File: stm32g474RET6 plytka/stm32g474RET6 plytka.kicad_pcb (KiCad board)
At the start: 4 copper layers, 73.5 x 39 mm, 60 parts, among them IC1 STM32G484RET6, IC2 SN65HVD230DR, IC3 SN65HVD230DR, IC4 TPSM63603V3RDHR, IC5 ESP32-S3-WROOM-1-N8, J1 5055670431, J2 5055670631, J3 5055670631, J4 5055670631, SW1 SW_Push, SW2 SW_Push, SW3 SW_Push

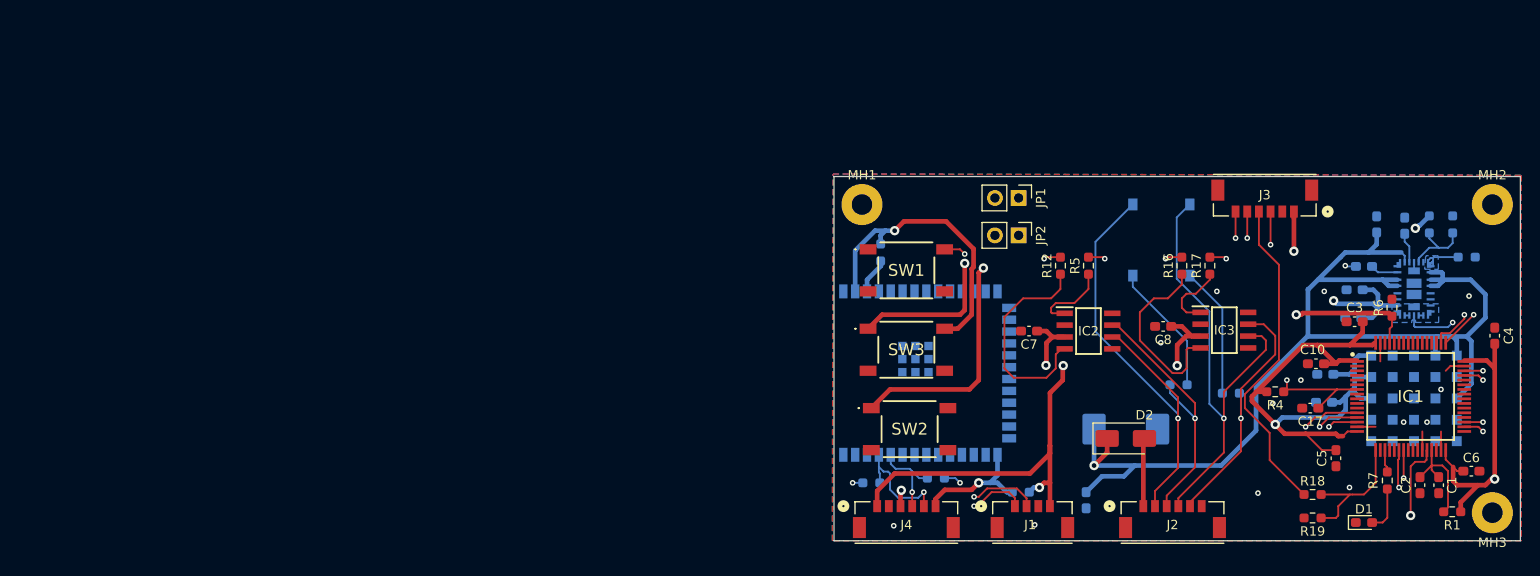
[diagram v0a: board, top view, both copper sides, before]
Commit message: added test points
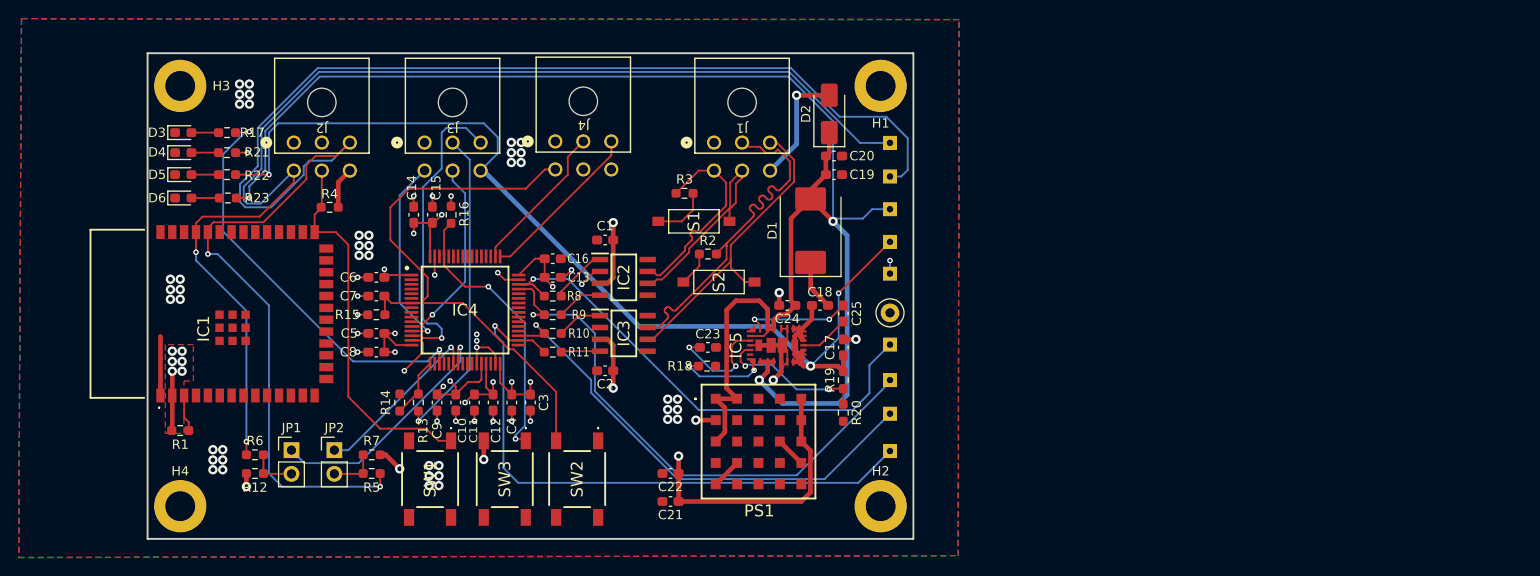
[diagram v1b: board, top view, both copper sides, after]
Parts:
- removed MH1, MH2, MH3: MountingHole_2.2mm_M2_Pad, MountingHole:MountingHole_2.2mm_M2_Pad
- added 12V1: TestPoint, TestPoint:TestPoint_THTPad_1.5x1.5mm_Drill0.7mm, B.Cu at (201.0, 122.7)
- added 3.3V1: TestPoint, TestPoint:TestPoint_THTPad_1.5x1.5mm_Drill0.7mm, B.Cu at (201.0, 129.6)
- added 5V1: TestPoint, TestPoint:TestPoint_THTPad_1.5x1.5mm_Drill0.7mm, B.Cu at (201.0, 126.2)
- added C14: 100n, Capacitor_SMD:C_0603_1608Metric_Pad1.08x0.95mm_HandSolder, F.Cu at (150.0, 123.3)
- added C20: 100u, Capacitor_SMD:C_0603_1608Metric_Pad1.08x0.95mm_HandSolder, F.Cu at (195.0, 117.0)
- added C22: 100n, Capacitor_SMD:C_0603_1608Metric_Pad1.08x0.95mm_HandSolder, F.Cu at (177.5, 151.0)
- added C23: 1u, Capacitor_SMD:C_0603_1608Metric_Pad1.08x0.95mm_HandSolder, F.Cu at (181.5, 137.5)
- added C24: 1u, Capacitor_SMD:C_0603_1608Metric_Pad1.08x0.95mm_HandSolder, F.Cu at (190.0, 133.0)
- added C25: 100n, Capacitor_SMD:C_0603_1608Metric_Pad1.08x0.95mm_HandSolder, F.Cu at (196.0, 133.9)
- added C9: 1u, Capacitor_SMD:C_0603_1608Metric_Pad1.08x0.95mm_HandSolder, F.Cu at (152.5, 143.4)
- added CAN1H1: TestPoint, TestPoint:TestPoint_THTPad_1.5x1.5mm_Drill0.7mm, B.Cu at (201.0, 141.0)
- added CAN1L1: TestPoint, TestPoint:TestPoint_THTPad_1.5x1.5mm_Drill0.7mm, B.Cu at (201.0, 137.2)
- added CAN2H1: TestPoint, TestPoint:TestPoint_THTPad_1.5x1.5mm_Drill0.7mm, B.Cu at (201.0, 148.6)
- added CAN2L1: TestPoint, TestPoint:TestPoint_THTPad_1.5x1.5mm_Drill0.7mm, B.Cu at (201.0, 144.6)
- added D4: LED, LED_SMD:LED_0603_1608Metric_Pad1.05x0.95mm_HandSolder, F.Cu at (125.3, 116.6)
- added D5: LED, LED_SMD:LED_0603_1608Metric_Pad1.05x0.95mm_HandSolder, F.Cu at (125.3, 119.0)
- added D6: LED, LED_SMD:LED_0603_1608Metric_Pad1.05x0.95mm_HandSolder, F.Cu at (125.3, 121.5)
- added GND1: TestPoint, TestPoint:TestPoint_Loop_D2.50mm_Drill1.0mm, F.Cu at (201.0, 133.8)
- added H1: MountingHole_Pad, MountingHole:MountingHole_3.2mm_M3_DIN965_Pad, F.Cu at (200.0, 109.5)
- added H2: MountingHole_Pad, MountingHole:MountingHole_3.2mm_M3_DIN965_Pad, F.Cu at (200.0, 154.5)
- added H3: MountingHole_Pad, MountingHole:MountingHole_3.2mm_M3_DIN965_Pad, F.Cu at (125.0, 109.5)
- added H4: MountingHole_Pad, MountingHole:MountingHole_3.2mm_M3_DIN965_Pad, F.Cu at (125.0, 154.5)
- added R20: 20k, Resistor_SMD:R_0603_1608Metric_Pad0.98x0.95mm_HandSolder, F.Cu at (196.0, 144.5)
- added R21: 330, Resistor_SMD:R_0603_1608Metric_Pad0.98x0.95mm_HandSolder, F.Cu at (130.0, 116.6)
- added R22: 1k, Resistor_SMD:R_0603_1608Metric_Pad0.98x0.95mm_HandSolder, F.Cu at (130.0, 119.0)
- added R23: 4.7k, Resistor_SMD:R_0603_1608Metric_Pad0.98x0.95mm_HandSolder, F.Cu at (130.1, 121.5)
- added RX1: TestPoint, TestPoint:TestPoint_THTPad_1.5x1.5mm_Drill0.7mm, B.Cu at (201.0, 119.2)
- added TX1: TestPoint, TestPoint:TestPoint_THTPad_1.5x1.5mm_Drill0.7mm, B.Cu at (201.0, 115.6)
- C11, C12, C15, C16, C19, PS1, R13, R2, R3, S1, S2: moved to F.Cu
- C13: value 22u -> 100n; moved to F.Cu
- C17: value 100n -> 22u
- C18: value 10u -> 100n; moved to F.Cu
- C2: value 1u -> 100n
- C21: value 1u -> 10u; moved to F.Cu
- D1: value LED -> D_TVS; footprint LED_SMD:LED_0603_1608Metric_Pad1.05x0.95mm_HandSolder -> Diode_SMD:D_SMC
- D3: value D_TVS -> LED; footprint Diode_SMD:D_SMC -> LED_SMD:LED_0603_1608Metric_Pad1.05x0.95mm_HandSolder; moved to F.Cu
- IC1: value STM32G484RET6 -> ESP32-S3-WROOM-1-N8; footprint Telemetry:QFP50P1200X1200X160-64N -> Telemetry:ESP32S3WROOM1N8R2
- IC4: value TPSM63603V3RDHR -> STM32G484RET6; footprint Telemetry:TPSM63603EXTRDHR -> Telemetry:QFP50P1200X1200X160-64N; moved to F.Cu
- IC5: value ESP32-S3-WROOM-1-N8 -> TPSM63603V3RDHR; footprint Telemetry:ESP32S3WROOM1N8R2 -> Telemetry:TPSM63603EXTRDHR; moved to F.Cu
- J1: value 5055670431 -> MicroFit+ 6pin; footprint Telemetry:CONN_505567_04_MOL -> Telemetry:CONN_2125280000_06_MOL
- J2, J3, J4: value 5055670631 -> MicroFit+ 6pin; footprint Telemetry:CONN_505567_06_MOL -> Telemetry:CONN_2125280000_06_MOL
- R1: value 10R -> 10k
- R10, R8: value 100k -> 100; moved to F.Cu
- R11: value 100R -> 100; moved to F.Cu
- R12, R5: value 100 -> 100R
- R14: value 10k -> 20k; moved to F.Cu
- R15: value 100R -> 10k; moved to F.Cu
- R16: value 100 -> 10k
- R17: value 100 -> 330R
- R18: value 10k -> 100k
- R19: value 20k -> 100k
- R6: value 10k -> 100R
- R7: value 330R -> 100R
- R9: value 20k -> 100; moved to F.Cu
- moved R1 136.5 mm to (125.0, 146.4), turned to 0 degrees
- moved IC1 128.9 mm to (128.1, 133.9), turned to 90 degrees
- moved R6 122.8 mm to (133.0, 149.0), turned to 180 degrees
- moved C6 119.1 mm to (146.0, 130.0), turned to 180 degrees
- moved R7 108.8 mm to (145.5, 149.0), turned to 180 degrees
- moved R17 106.2 mm to (130.0, 114.5), turned to 180 degrees
- moved D3 105.8 mm to (125.3, 114.5), turned to 0 degrees
- moved C4 105.5 mm to (160.5, 143.4), turned to -90 degrees
- moved C5 103.6 mm to (146.0, 136.0), turned to 180 degrees
- moved R4 103.2 mm to (141.0, 122.5), turned to 0 degrees
- moved J2 102.5 mm to (137.2, 115.6)
- moved IC4 101.6 mm to (155.5, 133.5), turned to 0 degrees
- moved C11 101.4 mm to (156.5, 143.4), turned to -90 degrees
- moved R10 98.2 mm to (164.9, 136.0)
- moved R9 96.8 mm to (164.9, 134.0), turned to 180 degrees
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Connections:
- C1 pad 1: Net-(IC1-VDDA) -> +3.3V
- C11 pad 1: Net-(IC4-VCC) -> +3.3V
- C12 pad 1: +5V -> +3.3V
- C13 pad 1: +5V -> +3.3V
- C15 pad 1: +12V -> +3.3V
- C16 pad 1: Net-(IC4-CBOOT) -> +3.3V
- C16 pad 2: Net-(IC4-SW) -> GND
- C17 pad 1: Net-(IC1-PG10-NRST) -> +5V
- C18 pad 1: +3.3V -> +5V
- C19 pad 1: +3.3V -> +12V
- C2 pad 1: Net-(IC1-VDDA) -> +3.3V
- C21 pad 1: +12V -> +3.3V
- C7 pad 1: +3.3V -> NRST
- D1 pad 2: Net-(D1-A) -> +12V
- D3 pad 2: +12V -> Net-(D3-A)
- IC1 pad 1: +3.3V -> GND
- IC1 pad 12: Net-(IC1-PA0) -> unconnected-(IC1-IO8-Pad12)
- IC1 pad 13: Net-(IC1-PA1) -> unconnected-(IC1-IO19-Pad13)
- IC1 pad 14: Net-(IC1-PA2) -> unconnected-(IC1-IO20-Pad14)
- IC1 pad 15: GND -> unconnected-(IC1-IO3-Pad15)
- IC1 pad 16: +3.3V -> unconnected-(IC1-IO46-Pad16)
- IC1 pad 17: Net-(IC1-PA3) -> unconnected-(IC1-IO9-Pad17)
- IC1 pad 19: Net-(IC1-PA5) -> unconnected-(IC1-IO11-Pad19)
- IC1 pad 2: unconnected-(IC1-PC13-Pad2) -> +3.3V
- IC1 pad 22: Net-(IC1-PC4) -> unconnected-(IC1-IO14-Pad22)
- IC1 pad 23: Net-(IC1-PC5) -> unconnected-(IC1-IO21-Pad23)
- IC1 pad 27: GND -> Net-(IC1-IO0)
- IC1 pad 28: +3.3V -> unconnected-(IC1-IO35-Pad28)
- IC1 pad 29: Net-(IC1-VDDA) -> unconnected-(IC1-IO36-Pad29)
- IC1 pad 3: (no net) -> Net-(IC1-EN)
- IC1 pad 31: GND -> unconnected-(IC1-IO38-Pad31)
- IC1 pad 32: +3.3V -> unconnected-(IC1-IO39-Pad32)
- IC1 pad 34: Net-(IC1-PB12) -> unconnected-(IC1-IO41-Pad34)
- IC1 pad 35: Net-(IC1-PB13) -> unconnected-(IC1-IO42-Pad35)
- IC1 pad 36: unconnected-(IC1-PB14-Pad36) -> Net-(IC1-RXD0)
- IC1 pad 37: unconnected-(IC1-PB15-Pad37) -> Net-(IC1-TXD0)
- IC1 pad 4: (no net) -> unconnected-(IC1-IO4-Pad4)
- IC1 pad 40: unconnected-(IC1-PC8-Pad40) -> GND
- IC1 pad 41: unconnected-(IC1-PC9-Pad41) -> GND
- IC1 pad 42: unconnected-(IC1-PA8-Pad42) -> GND
- IC1 pad 43: unconnected-(IC1-PA9-Pad43) -> GND
- IC1 pad 44: unconnected-(IC1-PA10-Pad44) -> GND
- IC1 pad 45: Net-(IC1-PA11) -> GND
- IC1 pad 46: Net-(IC1-PA12) -> GND
- IC1 pad 48: +3.3V -> GND
- IC1 pad 49: /SWCLK -> GND
- IC1 pad 6: (no net) -> unconnected-(IC1-IO6-Pad6)
- IC1 pad 7: Net-(IC1-PG10-NRST) -> unconnected-(IC1-IO7-Pad7)
- IC2 pad 4: +3.3V -> Net-(IC2-R)
- IC2 pad 6: Net-(IC2-CANL) -> /CAN_1_N
- IC2 pad 7: Net-(IC2-CANH) -> /CAN_1_P
- IC3 pad 4: +3.3V -> Net-(IC3-R)
- IC3 pad 6: Net-(IC3-CANL) -> /CAN_2_N
- IC3 pad 7: Net-(IC3-CANH) -> /CAN_2_P
- IC4 pad 1: Net-(IC4-RT_1) -> +3.3V
- IC4 pad 10: +5V -> unconnected-(IC4-PC2-Pad10)
- IC4 pad 11: Net-(IC4-SW) -> unconnected-(IC4-PC3-Pad11)
- IC4 pad 12: +5V -> Net-(IC4-PA0)
- IC4 pad 13: +5V -> Net-(IC4-PA1)
- IC4 pad 14: +5V -> Net-(IC4-PA2)
- IC4 pad 15: +5V -> GND
- IC4 pad 16: GND -> +3.3V
- IC4 pad 17: GND -> Net-(IC4-PA3)
- IC4 pad 18: +12V -> unconnected-(IC4-PA4-Pad18)
- IC4 pad 19: +12V -> Net-(IC4-PA5)
- IC4 pad 2: +12V -> unconnected-(IC4-PC13-Pad2)
- IC4 pad 20: Net-(IC4-CBOOT) -> unconnected-(IC4-PA6-Pad20)
- IC4 pad 22: +12V -> Net-(IC4-PC4)
- IC4 pad 23: Net-(IC4-VCC) -> Net-(IC4-PC5)
- IC4 pad 24: GND -> unconnected-(IC4-PB0-Pad24)
- IC4 pad 25: Net-(IC4-FB) -> unconnected-(IC4-PB1-Pad25)
- IC4 pad 28: GND -> +3.3V
- IC4 pad 29: GND -> +3.3V
- IC4 pad 3: +12V -> unconnected-(IC4-PC14-_OSC32_IN-Pad3)
- IC4 pad 30: +5V -> unconnected-(IC4-PB10-Pad30)
- IC4 pad 31: Net-(IC4-RT_1) -> GND
- IC4 pad 32: Net-(IC4-RT_1) -> +3.3V
- IC4 pad 33: +5V -> unconnected-(IC4-PB11-Pad33)
- IC4 pad 34: +5V -> Net-(IC4-PB12)
- IC4 pad 35: +5V -> Net-(IC4-PB13)
- IC4 pad 36: +5V -> unconnected-(IC4-PB14-Pad36)
- IC4 pad 4: +12V -> unconnected-(IC4-PC15-_OSC32_OUT-Pad4)
- IC4 pad 5: GND -> unconnected-(IC4-PF0-OSC_IN-Pad5)
- IC4 pad 6: GND -> unconnected-(IC4-PF1-_OSC_OUT-Pad6)
- IC4 pad 7: +5V -> NRST
- IC4 pad 8: +5V -> unconnected-(IC4-PC0-Pad8)
- IC4 pad 9: +5V -> unconnected-(IC4-PC1-Pad9)
- IC5 pad 10: unconnected-(IC5-IO17-Pad10) -> +5V
- IC5 pad 11: unconnected-(IC5-IO18-Pad11) -> Net-(IC5-SW)
- IC5 pad 12: unconnected-(IC5-IO8-Pad12) -> +5V
- IC5 pad 13: unconnected-(IC5-IO19-Pad13) -> +5V
- IC5 pad 15: unconnected-(IC5-IO3-Pad15) -> +5V
- IC5 pad 16: unconnected-(IC5-IO46-Pad16) -> GND
- IC5 pad 17: unconnected-(IC5-IO9-Pad17) -> GND
- IC5 pad 18: unconnected-(IC5-IO10-Pad18) -> +12V
- IC5 pad 19: unconnected-(IC5-IO11-Pad19) -> +12V
- IC5 pad 2: +3.3V -> +12V
- IC5 pad 20: unconnected-(IC5-IO12-Pad20) -> Net-(IC5-CBOOT)
- IC5 pad 22: unconnected-(IC5-IO14-Pad22) -> +12V
- IC5 pad 23: unconnected-(IC5-IO21-Pad23) -> Net-(IC5-VCC)
- IC5 pad 24: unconnected-(IC5-IO47-Pad24) -> GND
- IC5 pad 25: unconnected-(IC5-IO48-Pad25) -> Net-(IC5-FB)
- IC5 pad 27: Net-(IC5-IO0) -> GND
- IC5 pad 28: unconnected-(IC5-IO35-Pad28) -> GND
- IC5 pad 29: unconnected-(IC5-IO36-Pad29) -> GND
- IC5 pad 3: Net-(IC5-EN) -> +12V
- IC5 pad 30: unconnected-(IC5-IO37-Pad30) -> +5V
- IC5 pad 32: unconnected-(IC5-IO39-Pad32) -> Net-(IC5-RT_1)
- IC5 pad 33: unconnected-(IC5-IO40-Pad33) -> +5V
- IC5 pad 36: Net-(IC5-RXD0) -> +5V
- IC5 pad 37: Net-(IC5-TXD0) -> unconnected-(IC5-RBOOT_2-Pad37)_1
- IC5 pad 4: unconnected-(IC5-IO4-Pad4) -> +12V
- IC5 pad 5: unconnected-(IC5-IO5-Pad5) -> GND
- IC5 pad 6: unconnected-(IC5-IO6-Pad6) -> GND
- IC5 pad 7: unconnected-(IC5-IO7-Pad7) -> +5V
- IC5 pad 9: unconnected-(IC5-IO16-Pad9) -> +5V
- J1 pad 1: /SWCLK -> GND
- J1 pad 2: /SWDIO -> /CAN_2_P
- J1 pad 3: GND -> /CAN_2_N
- J1 pad 4: +3.3V -> /CAN_1_P
- J1 pad 5: (no net) -> /CAN_1_N
- J1 pad 6: (no net) -> Net-(D2-A)
- J2 pad 1: Net-(D2-A) -> GND
- J2 pad 2: Net-(IC2-CANL) -> +3.3V
- J2 pad 3: Net-(IC2-CANH) -> Net-(IC1-RXD0)
- J2 pad 4: Net-(IC3-CANL) -> Net-(IC1-TXD0)
- J2 pad 5: Net-(IC3-CANH) -> Net-(IC1-IO0)
- J2 pad 6: GND -> +3.3V
- J3 pad 1: +5V -> GND
- J3 pad 2: GND -> Net-(J3-Pad2)
- J3 pad 3: Net-(IC1-PA2) -> Net-(IC4-PA2)
- J3 pad 4: Net-(J3-Pad4) -> Net-(IC4-PA1)
- J3 pad 5: Net-(IC1-PA0) -> Net-(IC4-PA0)
- J3 pad 6: Net-(IC1-PA1) -> +5V
- J4 pad 1: +3.3V -> GND
- J4 pad 2: GND -> /SWDIO
- J4 pad 3: +3.3V -> /SWCLK
- J4 pad 4: Net-(IC5-RXD0) -> NRST
- J4 pad 5: Net-(IC5-TXD0) -> unconnected-(J4-Pad5)
- J4 pad 6: Net-(IC5-IO0) -> +3.3V
- JP1 pad 1: Net-(IC1-PC5) -> Net-(IC4-PC5)
- JP2 pad 1: Net-(IC1-PC4) -> Net-(IC4-PC4)
- R1 pad 2: Net-(IC1-VDDA) -> Net-(IC1-EN)
- R10 pad 1: GND -> Net-(IC3-D)
- R10 pad 2: Net-(IC4-RT_1) -> Net-(IC4-PB13)
- R11 pad 1: Net-(JP2-B) -> Net-(IC3-R)
- R11 pad 2: Net-(IC5-RXD0) -> Net-(IC4-PB12)
- R12 pad 2: Net-(IC1-PA11) -> Net-(JP1-B)
- R13 pad 1: +3.3V -> Net-(J3-Pad2)
- R13 pad 2: Net-(IC5-EN) -> Net-(IC4-PA3)
- R14 pad 1: Net-(IC5-IO0) -> Net-(IC4-PA3)
- R14 pad 2: +3.3V -> GND
- R15 pad 1: Net-(JP1-B) -> NRST
- R15 pad 2: Net-(IC5-TXD0) -> +3.3V
- R16 pad 1: +3.3V -> Net-(IC4-PB8-BOOT0)
- R16 pad 2: Net-(IC1-PB12) -> GND
- R17 pad 1: Net-(IC3-D) -> Net-(IC4-PA5)
- R17 pad 2: Net-(IC1-PB13) -> Net-(D3-A)
- R18 pad 1: Net-(J3-Pad4) -> GND
- R18 pad 2: Net-(IC1-PA3) -> Net-(IC5-RT_1)
- R19 pad 1: Net-(IC1-PA3) -> Net-(IC5-FB)
- R19 pad 2: GND -> +5V
- R2 pad 1: Net-(S1-COM) -> /CAN_2_Term
- R2 pad 2: Net-(IC2-CANH) -> /CAN_2_P
- R3 pad 1: Net-(S2-COM) -> /CAN_1_Term
- R3 pad 2: Net-(IC3-CANH) -> /CAN_1_P
- R4 pad 1: Net-(IC1-PG10-NRST) -> Net-(IC1-IO0)
- R5 pad 1: Net-(IC2-D) -> Net-(JP2-B)
- R5 pad 2: Net-(IC1-PA12) -> Net-(IC1-RXD0)
- R6 pad 1: Net-(IC1-PB8-BOOT0) -> Net-(JP1-B)
- R6 pad 2: GND -> Net-(IC1-TXD0)
- R7 pad 1: Net-(IC1-PA5) -> +3.3V
- R7 pad 2: Net-(D1-A) -> Net-(JP2-B)
- R8 pad 1: Net-(IC4-FB) -> Net-(IC2-D)
- R8 pad 2: +5V -> Net-(IC4-PA12)
- R9 pad 1: Net-(IC4-FB) -> Net-(IC2-R)
- R9 pad 2: GND -> Net-(IC4-PA11)
- S1 pad 1: Net-(S1-COM) -> /CAN_1_Term
- S1 pad 2: Net-(IC2-CANL) -> /CAN_1_N
- S2 pad 1: Net-(S2-COM) -> /CAN_2_Term
- S2 pad 2: Net-(IC3-CANL) -> /CAN_2_N
- SW1 pad 1: GND -> Net-(IC1-IO0)
- SW1 pad 2: Net-(IC1-PG10-NRST) -> GND
- SW2 pad 1: Net-(IC5-IO0) -> GND
- SW2 pad 2: GND -> NRST
- SW3 pad 1: Net-(IC1-PB8-BOOT0) -> Net-(IC4-PB8-BOOT0)
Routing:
- net +3.3V: track 347.9 -> 118.0 mm, vias 9 -> 27
- net Net-(IC1-RXD0): track 0.00 -> 168.9 mm, vias 0 -> 2
- net Net-(IC1-TXD0): track 0.00 -> 128.9 mm, vias 0 -> 2
- net Net-(IC1-PC5): track 77.5 -> 0.00 mm, vias 1 -> 0
- net Net-(IC1-PA11): track 75.5 -> 0.00 mm, vias 2 -> 0
- net +5V: track 42.5 -> 116.6 mm
- net Net-(IC1-PC4): track 71.4 -> 0.00 mm, vias 1 -> 0
- net Net-(IC1-PB8-BOOT0): track 68.0 -> 0.00 mm, vias 2 -> 0
- net Net-(IC1-PB12): track 67.6 -> 0.00 mm, vias 2 -> 0
- net Net-(IC1-PA12): track 67.2 -> 0.00 mm, vias 2 -> 0
- net /SWDIO: track 82.1 -> 16.2 mm, vias 2 -> 0
- net Net-(IC4-PB12): track 0.00 -> 65.5 mm, vias 0 -> 1
- net /SWCLK: track 81.3 -> 17.9 mm, vias 2 -> 0
- net NRST: track 0.00 -> 62.4 mm
- net Net-(IC5-IO0): track 61.6 -> 0.00 mm, vias 2 -> 0
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- added copper zone on F.Cu, net +3.3V
- added copper zone on In2.Cu, net +3.3V
- added copper zone on In1.Cu, net GND
- removed copper zone on B.Cu, net +5V
- removed copper zone on B.Cu, net Net-(IC4-RT_1)
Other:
- board size 73.5 x 39 mm -> 82 x 52 mm
